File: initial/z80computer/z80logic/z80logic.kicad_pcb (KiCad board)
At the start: 2 copper layers, 122.8 x 113.3 mm, 3 parts, among them J1 pin header 855-M20-9953645, J2 Conn_02x03_Top_Bottom

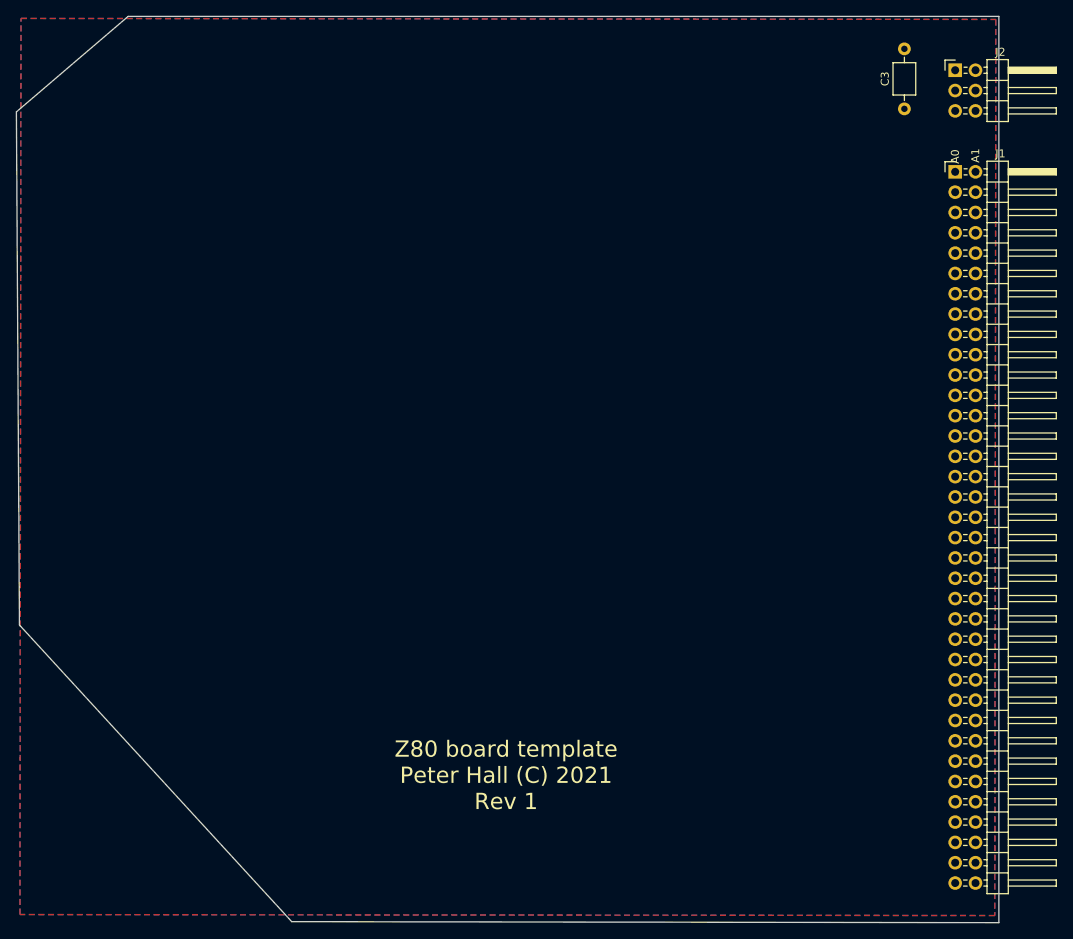
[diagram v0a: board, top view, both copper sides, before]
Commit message: version 1 circuit boards
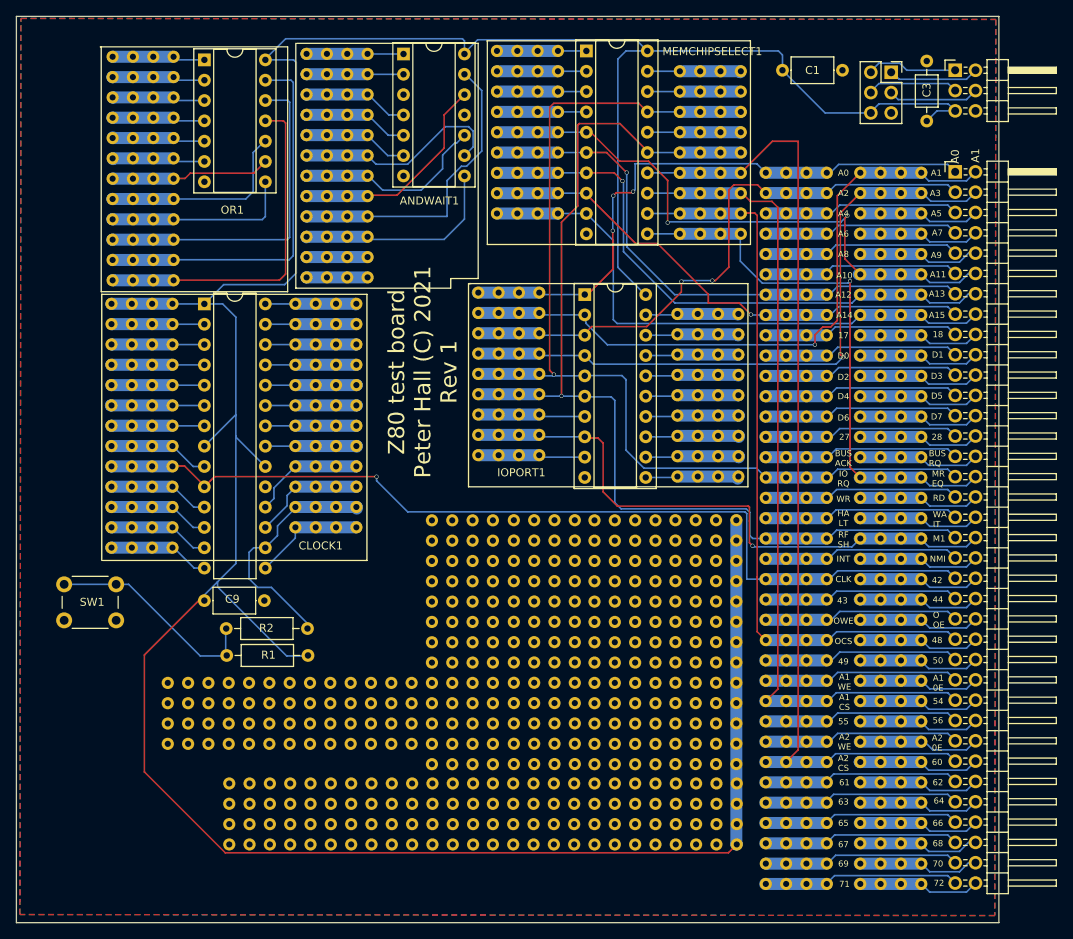
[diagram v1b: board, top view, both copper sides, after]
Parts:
- added ANDWAIT1: SN74HC21N, Package_DIP:DIP-14_W7.62mm_Socket, F.Cu at (165.0, 25.0)
- added C1: 0.1uF, Capacitor_THT:C_Axial_L5.1mm_D3.1mm_P7.50mm_Horizontal, F.Cu at (212.3, 27.1)
- added C10: perf_12x4symbol, circuit_boards:perf_12x4, F.Cu at (156.6, 34.0)
- added C11: perf_12x4symbol, circuit_boards:perf_12x4, F.Cu at (132.3, 34.4)
- added C12: perf_9x4symbol, circuit_boards:perf_9x4, F.Cu at (178.1, 63.9)
- added C13: perf_9x4symbol, circuit_boards:perf_9x4, F.Cu at (202.9, 66.5)
- added C14: perf_13x4symbol, circuit_boards:perf_13x4, F.Cu at (202.7, 92.3)
- added C15: perf_13x4symbol, circuit_boards:perf_13x4, F.Cu at (192.6, 92.3)
- added C16: perf_13x4symbol, circuit_boards:perf_13x4, F.Cu at (182.5, 92.3)
- added C17: perf_13x4symbol, circuit_boards:perf_13x4, F.Cu at (185.2, 120.1)
- added C18: perf_13x4symbol, circuit_boards:perf_13x4, F.Cu at (172.3, 92.3)
- added C19: perf_13x4symbol, circuit_boards:perf_13x4, F.Cu at (152.2, 120.1)
- added C2: perf_9x4symbol, circuit_boards:perf_9x4, F.Cu at (180.4, 33.7)
- added C20: perf_13x4symbol, circuit_boards:perf_13x4, F.Cu at (157.0, 107.4)
- added C4: perf_9x4symbol, circuit_boards:perf_9x4, F.Cu at (203.2, 36.2)
- added C5: perf_13x4symbol, circuit_boards:perf_13x4, F.Cu at (132.2, 65.3)
- added C6: perf_12x4symbol, circuit_boards:perf_12x4, F.Cu at (155.2, 65.3)
- added C7: perf_36x4symbol, circuit_boards:perf_36x4, F.Cu at (214.0, 48.9)
- added C8: perf_36x4symbol, circuit_boards:perf_36x4, F.Cu at (225.8, 48.9)
- added C9: 0.1uF, Capacitor_THT:C_Axial_L5.1mm_D3.1mm_P7.50mm_Horizontal, F.Cu at (140.1, 93.3)
- added CLOCK1: PIC18F24Q10-xSP, Package_DIP:DIP-28_W7.62mm, F.Cu at (140.1, 56.3)
- added IOPORT1: GAL16V8, Package_DIP:DIP-20_W7.62mm_Socket, F.Cu at (187.6, 55.1)
- added J3: Conn_02x03_Odd_Even, Connector_PinSocket_2.54mm:PinSocket_2x03_P2.54mm_Vertical, F.Cu at (225.9, 27.3)
- added MEMCHIPSELECT1: MEMCHIPSELECT, Package_DIP:DIP-20_W7.62mm_Socket, F.Cu at (187.8, 24.6)
- added OR1: SN74LS32N, Package_DIP:DIP-14_W7.62mm_Socket, F.Cu at (140.1, 25.8)
- added R1: 1K, Resistor_THT:R_Axial_DIN0207_L6.3mm_D2.5mm_P10.16mm_Horizontal, F.Cu at (142.9, 100.2)
- added R2: 1K, Resistor_THT:R_Axial_DIN0207_L6.3mm_D2.5mm_P10.16mm_Horizontal, F.Cu at (142.8, 96.8)
- added SW1: SW_SPST, Button_Switch_THT:SW_PUSH_6mm_H8mm, F.Cu at (122.6, 91.3)
- moved C3 3.18 mm to (230.4, 33.4)
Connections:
- J1 pad 17: Net-(J1-Pad17) -> /17
- J1 pad 18: Net-(J1-Pad18) -> /18
- J1 pad 27: Net-(J1-Pad27) -> /27
- J1 pad 28: Net-(J1-Pad28) -> /28
- J1 pad 42: Net-(J1-Pad42) -> /42
- J1 pad 43: Net-(J1-Pad43) -> /43
- J1 pad 44: Net-(J1-Pad44) -> /44
- J1 pad 48: Net-(J1-Pad48) -> /48
- J1 pad 49: Net-(J1-Pad49) -> /49
- J1 pad 50: Net-(J1-Pad50) -> /50
- J1 pad 54: Net-(J1-Pad54) -> /54
- J1 pad 55: Net-(J1-Pad55) -> /55
- J1 pad 56: Net-(J1-Pad56) -> /56
- J1 pad 60: Net-(J1-Pad60) -> /60
- J1 pad 61: Net-(J1-Pad61) -> /61
- J1 pad 62: Net-(J1-Pad62) -> /62
- J1 pad 63: Net-(J1-Pad63) -> /63
- J1 pad 64: Net-(J1-Pad64) -> /64
- J1 pad 65: Net-(J1-Pad65) -> /65
- J1 pad 66: Net-(J1-Pad66) -> /66
- J1 pad 67: Net-(J1-Pad67) -> /67
- J1 pad 68: Net-(J1-Pad68) -> /68
- J1 pad 69: Net-(J1-Pad69) -> /69
- J1 pad 70: Net-(J1-Pad70) -> /70
- J1 pad 71: Net-(J1-Pad71) -> /71
- J1 pad 72: Net-(J1-Pad72) -> /72
- J2 pad 2: Net-(J2-Pad2) -> /POWER2
- J2 pad 3: Net-(J2-Pad3) -> /POWER3
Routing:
- net /VCC5: track 0.00 -> 401.6 mm
- net /RFSH: track 0.00 -> 133.3 mm, vias 0 -> 1
- net /IORQ: track 0.00 -> 128.6 mm, vias 0 -> 1
- net /A2CS: track 0.00 -> 123.1 mm
- net /CLK: track 0.00 -> 118.0 mm, vias 0 -> 1
- net /A1CS: track 0.00 -> 103.6 mm
- net /OCS: track 0.00 -> 91.4 mm
- net /A1: track 0.00 -> 83.7 mm, vias 0 -> 1
- net /A3: track 0.00 -> 83.4 mm, vias 0 -> 1
- net /A11: track 0.00 -> 75.8 mm, vias 0 -> 2
- net /M1: track 0.00 -> 75.5 mm, vias 0 -> 1
- net /A0: track 0.00 -> 74.7 mm, vias 0 -> 3
- net /A2: track 0.00 -> 74.3 mm, vias 0 -> 2
- net /A13: track 0.00 -> 72.9 mm, vias 0 -> 1
- net /A15: track 0.00 -> 72.8 mm
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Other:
- outline, holes or cut-outs redrawn
- board text added: "03A"
- board text added: "03B"
- board text added: "1"
- board text added: "11"
- board text added: "12"
- board text added: "13"
- board text added: "14"
- board text added: "15"
- board text added: "16"
- board text added: "17"
- board text added: "18"
- board text added: "19"
- board text added: "2"
- board text added: "21"
- board text added: "22"
- board text added: "23"
- board text added: "24"
- board text added: "25"
- board text added: "26"
- board text added: "27"
- board text added: "28"
- board text added: "3"
- board text added: "4"
- board text added: "42"
- board text added: "43"
- board text added: "44"
- board text added: "48"
- board text added: "49"
- board text added: "5"
- board text added: "50"
- board text added: "54"
- board text added: "55"
- board text added: "56"
- board text added: "6"
- board text added: "60"
- board text added: "61"
- board text added: "62"
- board text added: "63"
- board text added: "64"
- board text added: "65"
- board text added: "66"
- board text added: "67"
- board text added: "68"
- board text added: "69"
- board text added: "7"
- board text added: "70"
- board text added: "71"
- board text added: "72"
- board text added: "9"
- board text added: "A1 0E"
- board text added: "A1 CS"
- board text added: "A1 WE"
- board text added: "A10"
- board text added: "A11"
- board text added: "A12"
- board text added: "A13"
- board text added: "A14"
- board text added: "A15"
- board text added: "A1A"
- board text added: "A1B"
- board text added: "A1C"
- board text added: "A1CS"
- board text added: "A1D"
- board text added: "A1Y"
- board text added: "A2"
- board text added: "A2 0E"
- board text added: "A2 CS"
- board text added: "A2 WE"
- board text added: "A2A"
- board text added: "A2B"
- board text added: "A2C"
- board text added: "A2CS"
- board text added: "A2D"
- board text added: "A2Y"
- board text added: "A3"
- board text added: "A4"
- board text added: "A5"
- board text added: "A6"
- board text added: "A7"
- board text added: "A8"
- board text added: "A9"
- board text added: "BUS ACK"
- board text added: "BUS RQ"
- board text added: "CLK"
- board text added: "D0"
- board text added: "D1"
- board text added: "D2"
- board text added: "D3"
- board text added: "D4"
- board text added: "D5"
- board text added: "D6"
- board text added: "D7"
- board text added: "HA LT"
- board text added: "INT"
- board text added: "IO RQ"
- board text added: "IORQ"
- board text added: "M1"
- board text added: "MR EQ"
- board text added: "MREQ"
- board text added: "NMI"
- board text added: "O OE"
- board text added: "O1A"
- board text added: "O1B"
- board text added: "O1Y"
- board text added: "O2A"
- board text added: "O2B"
- board text added: "O2Y"
- board text added: "O3Y"
- board text added: "O4A"
- board text added: "O4B"
- board text added: "O4Y"
- board text added: "OCS"
- board text added: "OWE"
- board text added: "RD"
- board text added: "RF SH"
- board text added: "RFSH"
- board text added: "VCC5"
- board text added: "WA IT"
- board text added: "WR"
- board text added: "Z80 test board Peter Hall (C) 2021 Rev 1"
- board text removed: "A1-A0"
- board text removed: "A10E-A1WE"
- board text removed: "A11-A10"
- board text removed: "A13-A12"
- board text removed: "A15-A14"
- board text removed: "A20E-A2WE"
- board text removed: "A3-A2"
- board text removed: "A5-A4"
- board text removed: "A7-A6"
- board text removed: "A9-A10"
- board text removed: "BUSRQ-BUSACK"
- board text removed: "D1-D0"
- board text removed: "D3-D2"
- board text removed: "D5-D4"
- board text removed: "D7-D6"
- board text removed: "M1-RFSH"
- board text removed: "MREQ-IORQ"
- board text removed: "NMI-INT"
- board text removed: "OOE-OWE"
- board text removed: "RD-WR"
- board text removed: "WAIT-HALT"
- board text removed: "Z80 board template Peter Hall (C) 2021 Rev 1"
- board text removed: "x-A1CS"
- board text removed: "x-A2CS"
- board text removed: "x-CLK"
- board text removed: "x-OCS"
